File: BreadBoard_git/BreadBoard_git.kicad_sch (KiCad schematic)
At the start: 36 parts, among them Q1 CSD18512Q5B, Q2 CSD18512Q5B, Q3 RQ3E110AJTB, Q4 RQ3E110AJTB, Q5 RQ3E110AJTB, U1 ESP32-S3, U2 LM73605RNPR, U3 LM5148RGYR

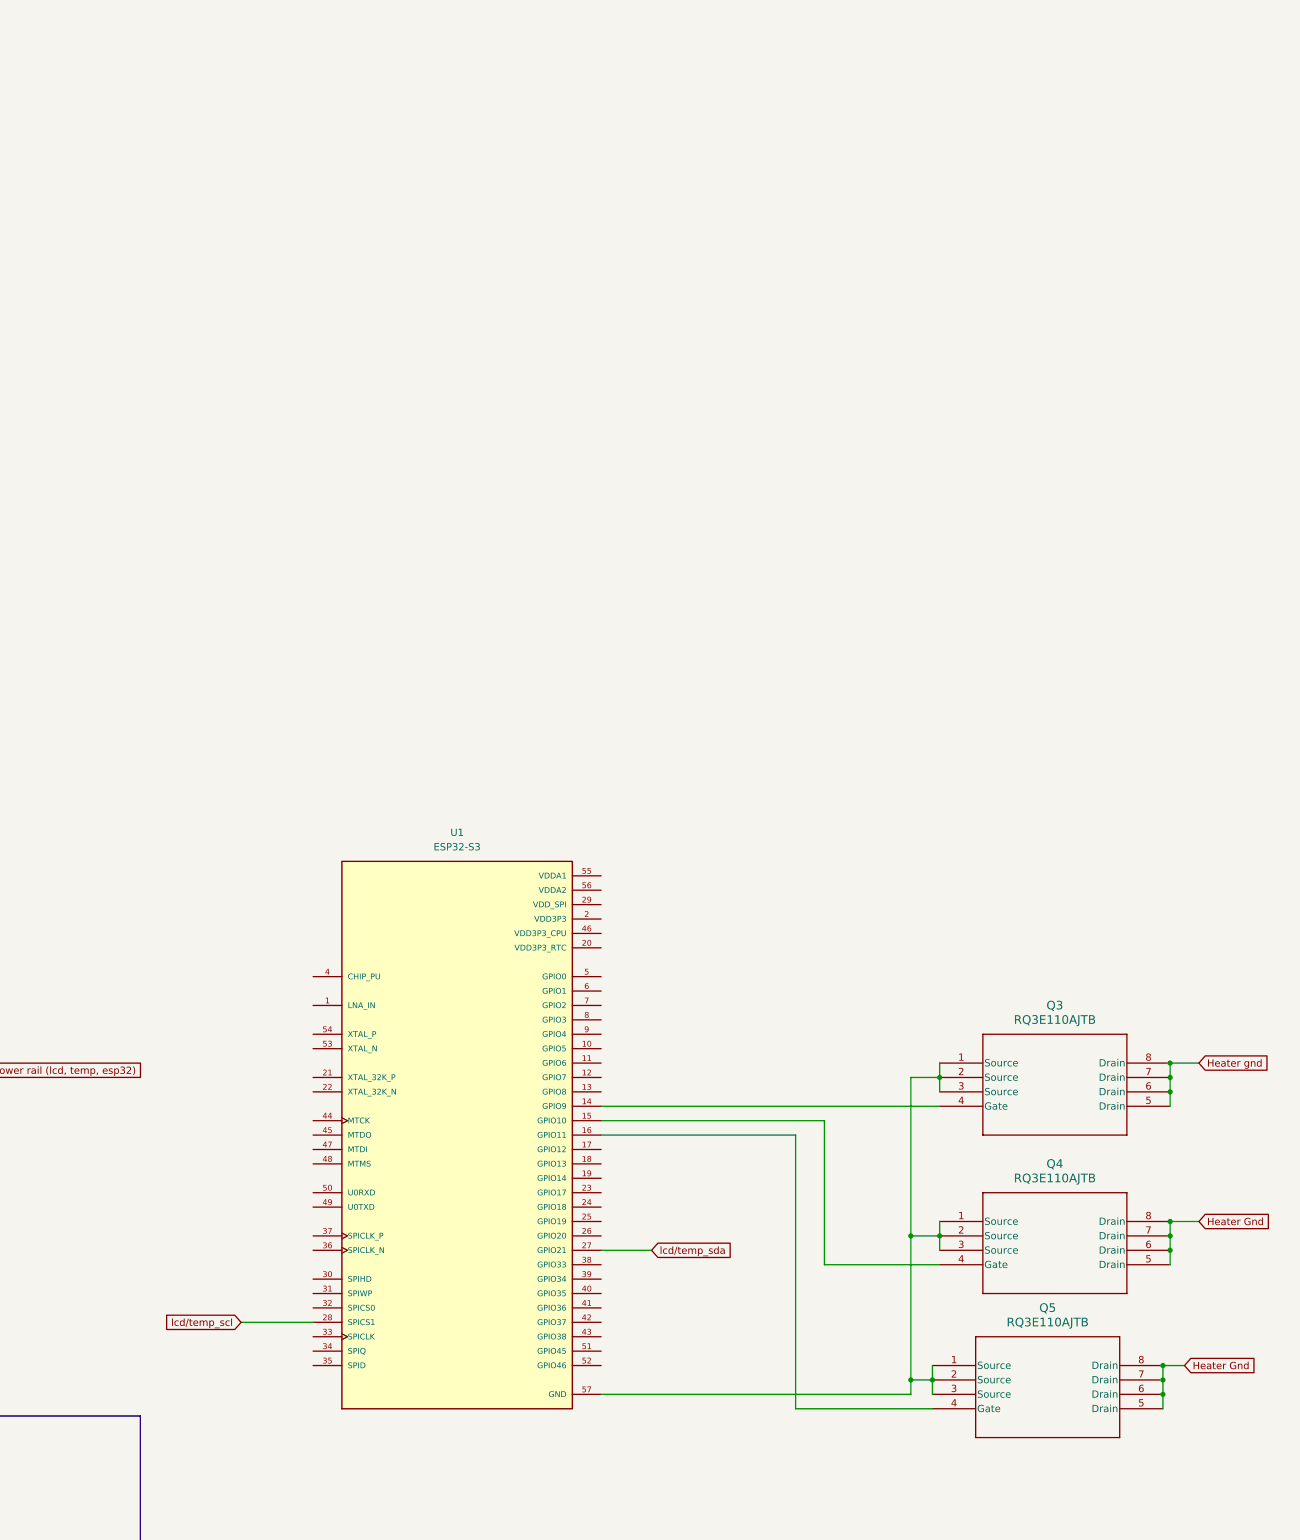
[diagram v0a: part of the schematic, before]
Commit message: update
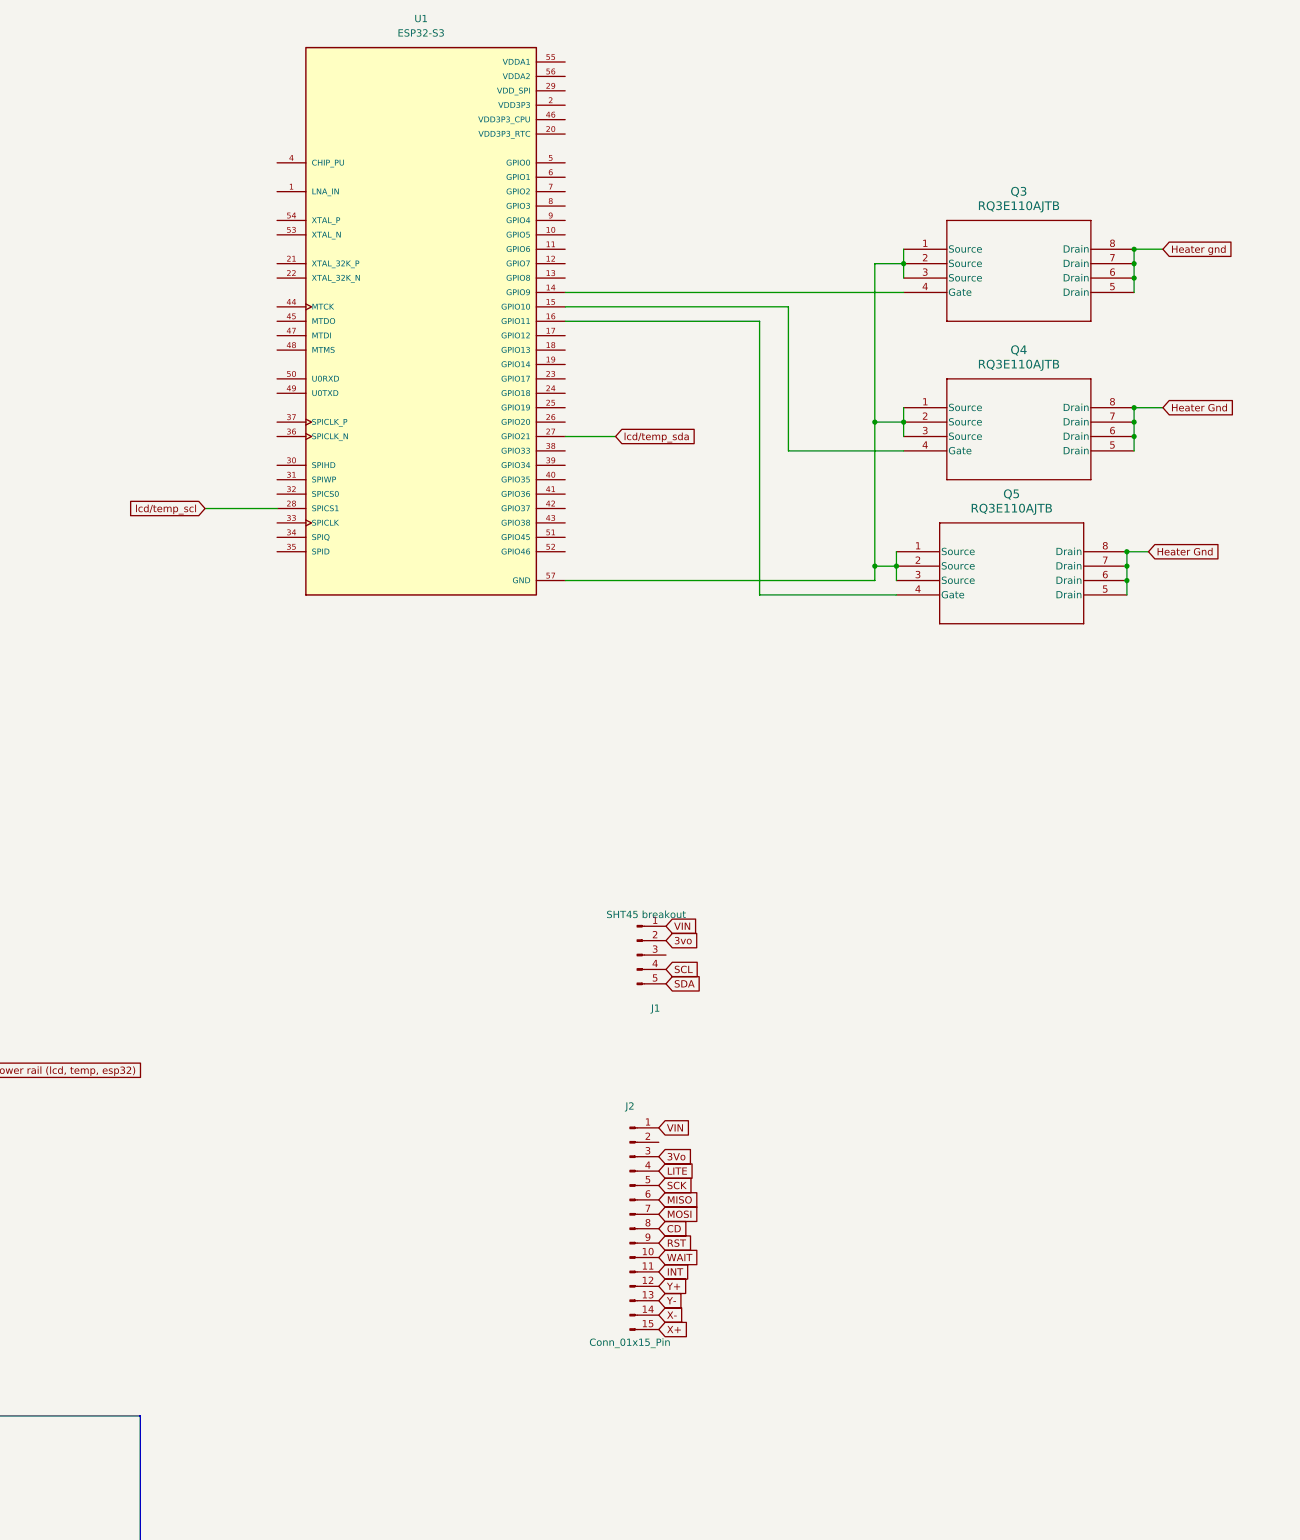
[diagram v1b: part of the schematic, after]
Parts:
- added J1: SHT45 breakout, symbol Connector:Conn_01x05_Pin
- added J2: Conn_01x15_Pin, symbol Connector:Conn_01x15_Pin
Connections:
- new net 3Vo: J2.3 (Pin_3)
- new net 3vo: J1.2 (Pin_2)
- new net CD: J2.8 (Pin_8)
- new net INT: J2.11 (Pin_11)
- new net LITE: J2.4 (Pin_4)
- new net MISO: J2.6 (Pin_6)
- new net MOSI: J2.7 (Pin_7)
- new net RST: J2.9 (Pin_9)
- new net SCK: J2.5 (Pin_5)
- new net SCL: J1.4 (Pin_4)
- new net SDA: J1.5 (Pin_5)
- new net VIN: J1.1 (VIN), J2.1 (Pin_1)
- new net WAIT: J2.10 (Pin_10)
- new net X+: J2.15 (Pin_15)
- new net X-: J2.14 (Pin_14)
- new net Y+: J2.12 (Pin_12)
- new net Y-: J2.13 (Pin_13)
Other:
- moved on the sheet: Q3, Q4, Q5, U1
